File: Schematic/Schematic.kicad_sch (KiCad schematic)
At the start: 23 parts, among them J1 STEP/DIR, J2 VCC_IO, J3 MISC

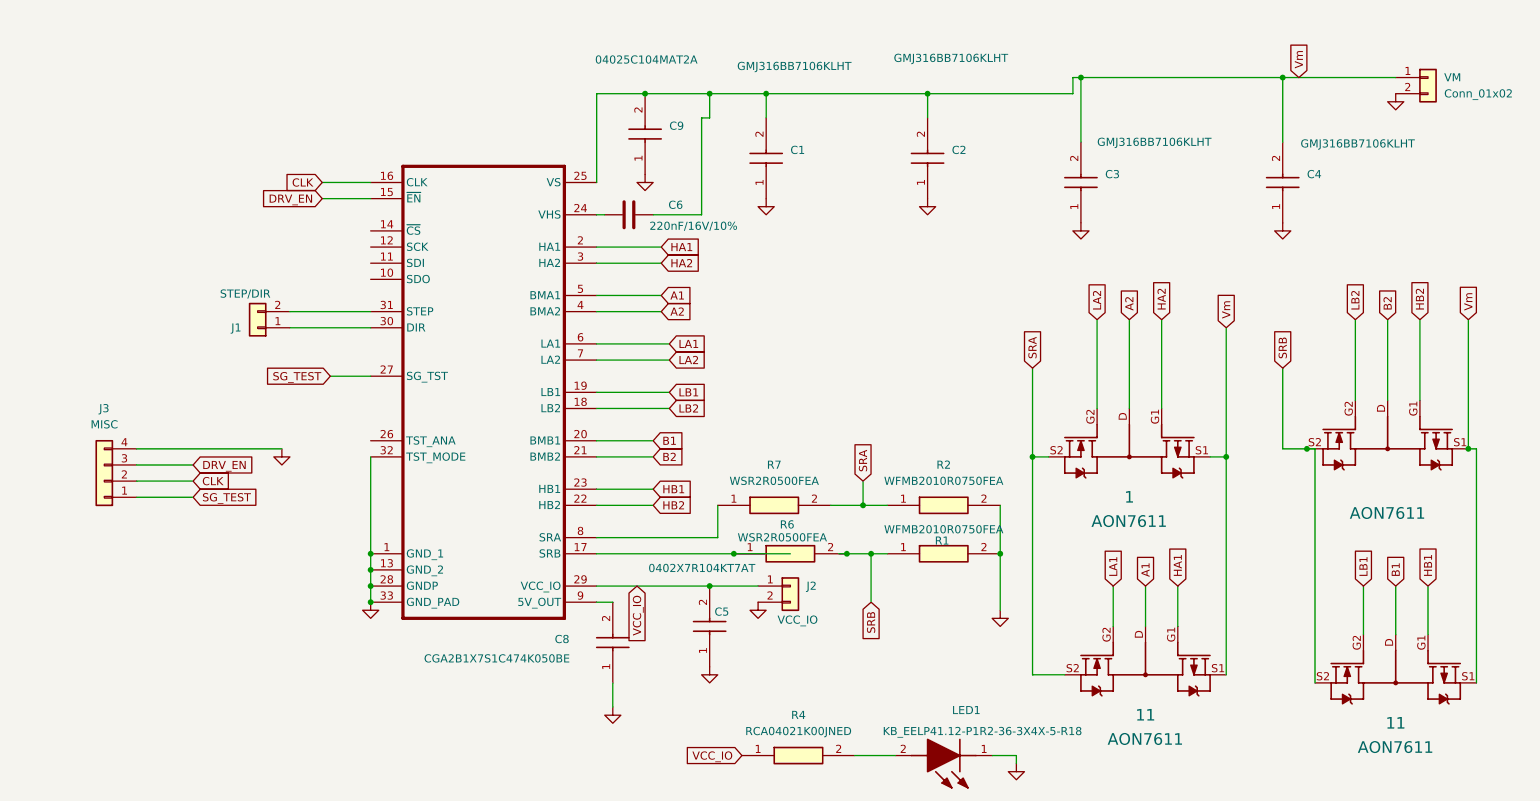
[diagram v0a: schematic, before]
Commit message: this is alot
good luck
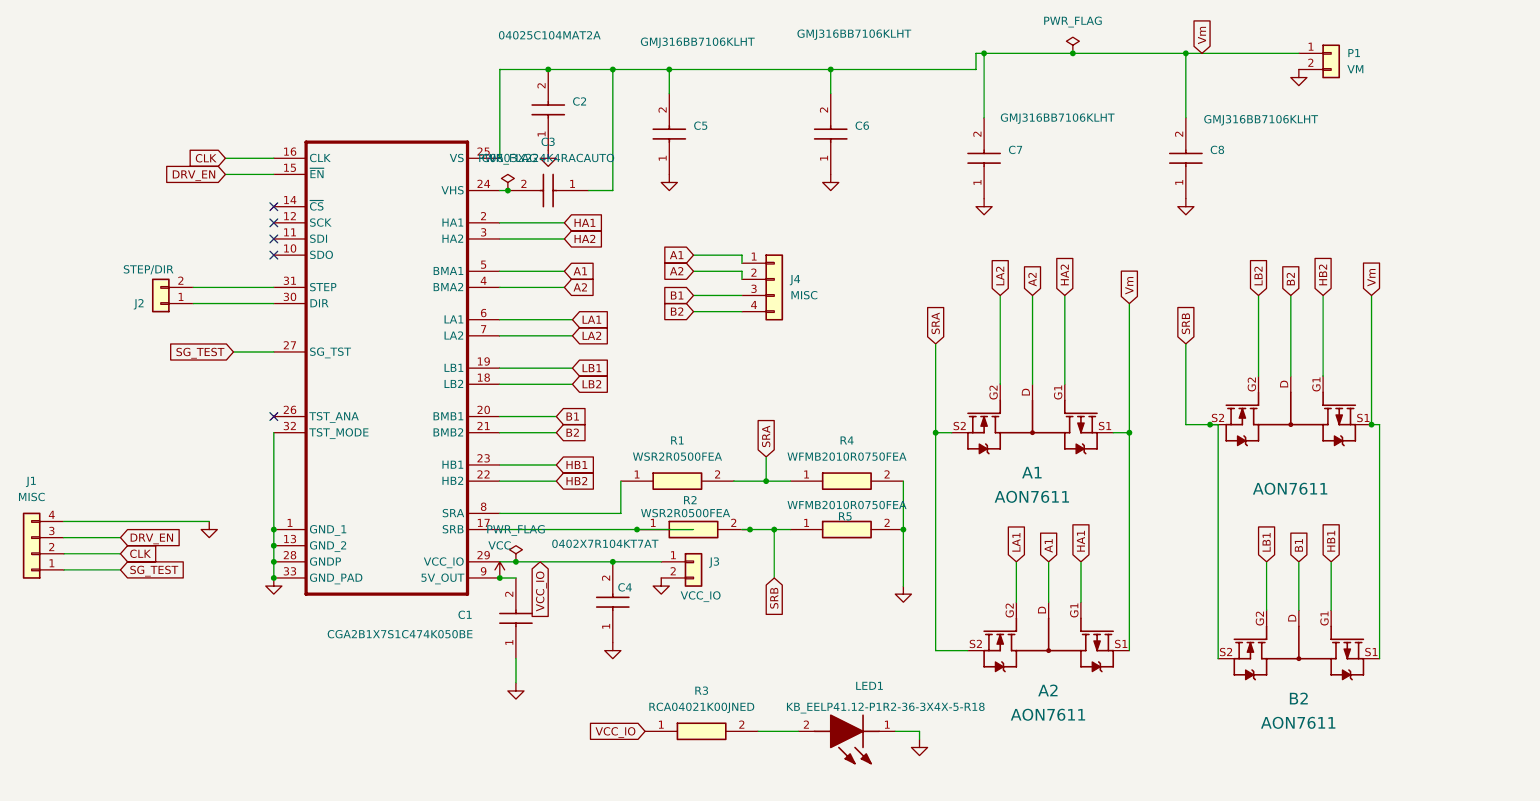
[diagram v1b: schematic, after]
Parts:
- removed 1, 11 (x3): AON7611, AON7611, symbol TMC262_BOB40_V1_2:AON7611
- removed C1, C2, C3, C4: GMJ316BB7106KLHT, CAPPC3216X125N, symbol GMJ316BB7106KLHT:GMJ316BB7106KLHT
- removed C5: 0402X7R104KT7AT, CAPC1005X61N, symbol 0402X7R104KT7AT:0402X7R104KT7AT
- removed C6: 220nF/16V/10%, 100nF/50V/20%, symbol Device:C
- removed C8: CGA2B1X7S1C474K050BE, CAPC1005X55N, symbol CGA2B1X7S1C474K050BE:CGA2B1X7S1C474K050BE
- removed C9: 04025C104MAT2A, CAPC1005X56N, symbol 04025C104MAT2A:04025C104MAT2A
- removed J1: STEP/DIR, symbol Connector_Generic:Conn_01x02
- removed J3: MISC, symbol Connector_Generic:Conn_01x04
- removed R1, R2: WFMB2010R0750FEA, RESC5125X65N, symbol WFMB2010R0750FEA:WFMB2010R0750FEA
- removed R4: RCA04021K00JNED, RESC1005X40N, symbol RCA04021K00JNED:RCA04021K00JNED
- removed R6, R7: WSR2R0500FEA, RESM11670X254N, symbol WSR2R0500FEA:WSR2R0500FEA
- removed VM: Conn_01x02, symbol Connector_Generic:Conn_01x02
- added A1, A2, B1, B2: AON7611, Package_SO:SOIC-8_3.9x4.9mm_P1.27mm, symbol TMC262_BOB40_V1_2:AON7611
- added C1: CGA2B1X7S1C474K050BE, Capacitor_SMD:C_0402_1005Metric, symbol CGA2B1X7S1C474K050BE:CGA2B1X7S1C474K050BE
- added C2: 04025C104MAT2A, Capacitor_SMD:C_0402_1005Metric, symbol 04025C104MAT2A:04025C104MAT2A
- added C3: C0603X224K4RACAUTO, Capacitor_SMD:C_0603_1608Metric, symbol C0603X224K4RACAUTO:C0603X224K4RACAUTO
- added C4: 0402X7R104KT7AT, Capacitor_SMD:C_0402_1005Metric, symbol 0402X7R104KT7AT:0402X7R104KT7AT
- added C5, C6, C7, C8: GMJ316BB7106KLHT, Capacitor_SMD:C_1206_3216Metric, symbol GMJ316BB7106KLHT:GMJ316BB7106KLHT
- added J1, J4: MISC, Connector_PinHeader_2.54mm:PinHeader_1x04_P2.54mm_Vertical, symbol Connector_Generic:Conn_01x04
- added J3: VCC_IO, Connector_PinHeader_2.54mm:PinHeader_1x02_P2.54mm_Vertical, symbol Connector_Generic:Conn_01x02
- added P1: VM, Connector_Phoenix_MSTB:PhoenixContact_MSTBA_2,5_2-G_1x02_P5.00mm_Horizontal, symbol Connector_Generic:Conn_01x02
- added R1, R2: WSR2R0500FEA, Resistor_SMD:R_Shunt_Vishay_WSR2_WSR3, symbol WSR2R0500FEA:WSR2R0500FEA
- added R3: RCA04021K00JNED, Resistor_SMD:R_0402_1005Metric, symbol RCA04021K00JNED:RCA04021K00JNED
- added R4, R5: WFMB2010R0750FEA, Resistor_SMD:R_2010_5025Metric, symbol WFMB2010R0750FEA:WFMB2010R0750FEA
- IC1: footprint TMC262-LA:TMC_QFN32_0.5_5.0X5.0 -> Package_DFN_QFN:QFN-32-1EP_5x5mm_P0.5mm_EP3.3x3.3mm_ThermalVias
- J2: value VCC_IO -> STEP/DIR; footprint (none) -> Connector_PinHeader_2.54mm:PinHeader_1x02_P2.54mm_Vertical
- LED1: footprint KBEELP4112P1R2363X4X5R18 -> LED_SMD:LED_0805_2012Metric
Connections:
- net A1: now also A2.D, J4.1 (Pin_1)
- net A2: now also A1.D, J4.2 (Pin_2)
- net B1: now also B2.D, J4.3 (Pin_3)
- net B2: now also B1.D, J4.4 (Pin_4)
- net CLK: now also J1.2 (Pin_2)
- net DRV_EN: now also J1.3 (Pin_3)
- net GND: now also C1.1, C2.1, C4.1, C5.1, C6.1, C7.1, C8.1, J1.4 (Pin_4), J3.2 (Pin_2), P1.2 (Pin_2), R4.2, R5.2; no longer J2.2 (Pin_2)
- net HA1: now also A2.G1
- net HA2: now also A1.G1
- net HB1: now also B2.G1
- net HB2: now also B1.G1
- net LA1: now also A2.G2
- net LA2: now also A1.G2
- net LB1: now also B2.G2
- net LB2: now also B1.G2
- net SG_TEST: now also J1.1 (Pin_1)
- net SRA: now also A1.S2, A2.S2, R1.2, R4.1
- net SRB: now also B1.S2, B2.S2, R2.2, R5.1
- net VCC_IO: now also C4.2, J3.1 (Pin_1), R3.1; no longer J2.1 (Pin_1)
- net Vm: now also A1.S1, A2.S1, B1.S1, B2.S1, C2.2, C3.1, C5.2, C6.2, C7.2, C8.2, P1.1 (Pin_1)
- net at IC1.24 (VHS): now also C3.2
- net at IC1.8 (SRA): now also R1.1
- net at IC1.17 (SRB): now also R2.1
- net at IC1.30 (DIR): now also J2.1 (Pin_1)
- net at IC1.31 (STEP): now also J2.2 (Pin_2)
- net VCC: now reaches IC1.9 (5V_OUT)
- net VCC: now also C1.2
- net at LED1.2 (A): now also R3.2
- no-connect marks 0 -> 5
